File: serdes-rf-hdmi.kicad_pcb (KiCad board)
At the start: 4 copper layers, 33.5 x 33 mm, 13 parts, among them J1 HDMI_A, J2 SMA, J3 SMA

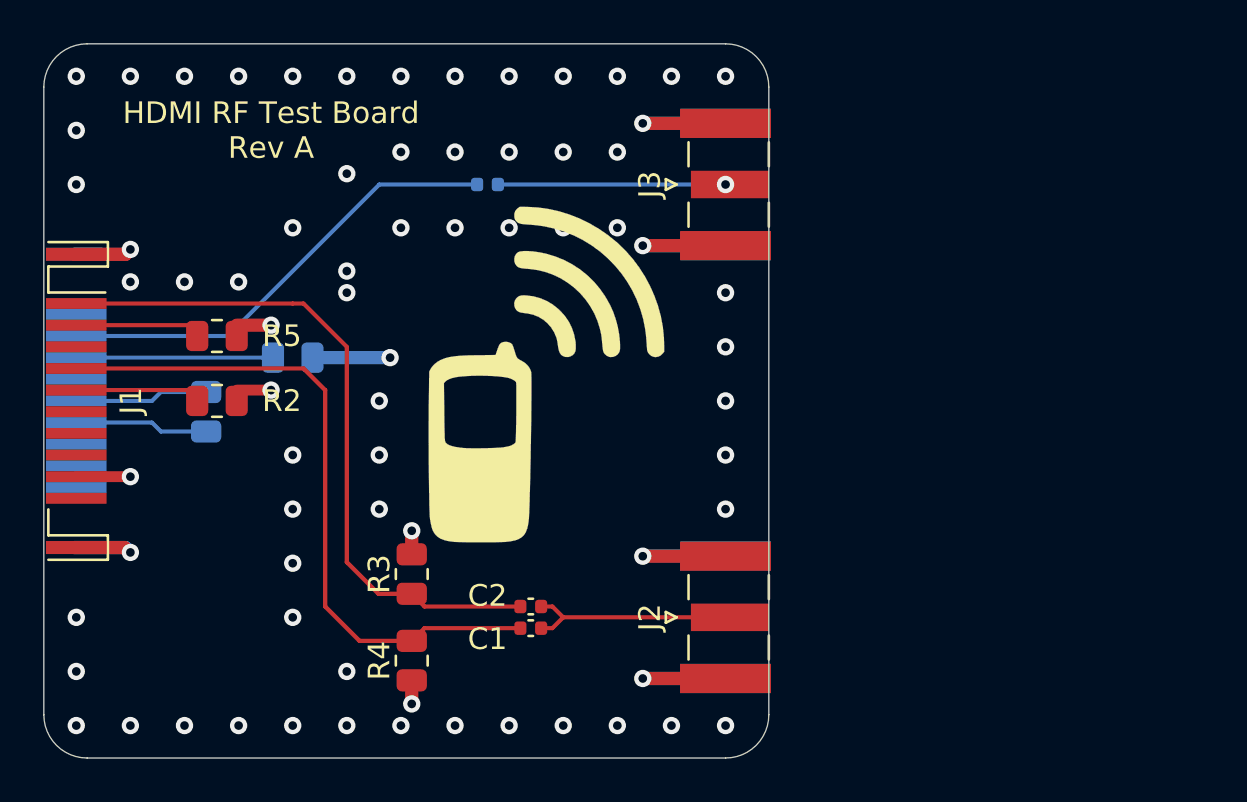
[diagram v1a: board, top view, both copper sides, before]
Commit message: Rev B complete
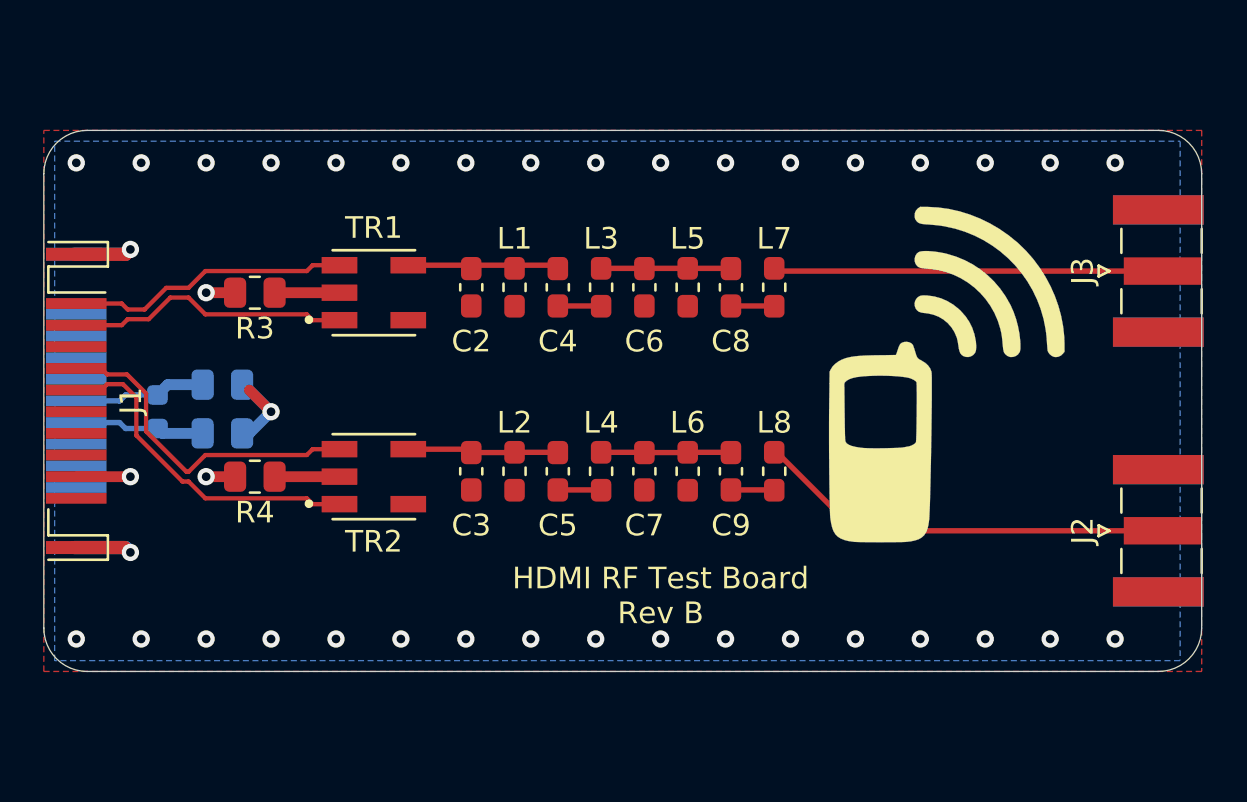
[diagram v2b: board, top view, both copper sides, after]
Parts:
- removed R5, R6: 50R, Resistor_SMD:R_0805_2012Metric
- added C4: 3.3pF, Capacitor_SMD:C_0603_1608Metric_Pad1.08x0.95mm_HandSolder, F.Cu at (142.2, 79.8)
- added C5: 3.3pF, Capacitor_SMD:C_0603_1608Metric_Pad1.08x0.95mm_HandSolder, F.Cu at (142.2, 88.2)
- added C6: 160pF, Capacitor_SMD:C_0603_1608Metric_Pad1.08x0.95mm_HandSolder, F.Cu at (146.2, 79.8)
- added C7: 160pF, Capacitor_SMD:C_0603_1608Metric_Pad1.08x0.95mm_HandSolder, F.Cu at (146.2, 88.2)
- added C8: 3.3pF, Capacitor_SMD:C_0603_1608Metric_Pad1.08x0.95mm_HandSolder, F.Cu at (150.2, 79.8)
- added C9: 3.3pF, Capacitor_SMD:C_0603_1608Metric_Pad1.08x0.95mm_HandSolder, F.Cu at (150.2, 88.2)
- added L1: 8.2nH, Inductor_SMD:L_0603_1608Metric_Pad1.05x0.95mm_HandSolder, F.Cu at (140.2, 79.8)
- added L2: 8.2nH, Inductor_SMD:L_0603_1608Metric_Pad1.05x0.95mm_HandSolder, F.Cu at (140.2, 88.2)
- added L3: 430nH, Inductor_SMD:L_0603_1608Metric_Pad1.05x0.95mm_HandSolder, F.Cu at (144.2, 79.8)
- added L4: 430nH, Inductor_SMD:L_0603_1608Metric_Pad1.05x0.95mm_HandSolder, F.Cu at (144.2, 88.2)
- added L5: 8.2nH, Inductor_SMD:L_0603_1608Metric_Pad1.05x0.95mm_HandSolder, F.Cu at (148.2, 79.8)
- added L6: 8.2nH, Inductor_SMD:L_0603_1608Metric_Pad1.05x0.95mm_HandSolder, F.Cu at (148.2, 88.2)
- added L7: 430nH, Inductor_SMD:L_0603_1608Metric_Pad1.05x0.95mm_HandSolder, F.Cu at (152.2, 79.8)
- added L8: 430nH, Inductor_SMD:L_0603_1608Metric_Pad1.05x0.95mm_HandSolder, F.Cu at (152.2, 88.2)
- added TR1: TC1-1TX+, serdes-rf-hdmi:XFMR_TC1-1-13M+, F.Cu at (133.8, 80.0)
- added TR2: TC1-1TX+, serdes-rf-hdmi:XFMR_TC1-1-13M+, F.Cu at (133.8, 88.5)
- C1: footprint Capacitor_SMD:C_0402_1005Metric -> Capacitor_SMD:C_0603_1608Metric; moved to B.Cu
- C2: value 10nF -> 160pF; footprint Capacitor_SMD:C_0402_1005Metric -> Capacitor_SMD:C_0603_1608Metric_Pad1.08x0.95mm_HandSolder
- C3: value 10nF -> 160pF; footprint Capacitor_SMD:C_0402_1005Metric -> Capacitor_SMD:C_0603_1608Metric_Pad1.08x0.95mm_HandSolder; moved to F.Cu
- R2: moved to B.Cu
- moved J2 25.6 mm to (170.0, 91.0)
- moved J3 25.6 mm to (170.0, 79.0)
- moved C1 19.9 mm to (123.8, 85.5), turned to 270 degrees
- moved G1 18.5 mm to (158.5, 84.0)
- moved C2 15.0 mm to (138.2, 79.8), turned to 270 degrees
- moved R3 14.9 mm to (128.2, 80.0), turned to 180 degrees
- moved C3 13.3 mm to (138.2, 88.2), turned to 270 degrees
- moved R4 11.2 mm to (128.2, 88.5), turned to 180 degrees
- moved R2 1.52 mm to (126.8, 86.5), turned to 180 degrees
- moved R1 1.46 mm to (126.8, 84.2), turned to 180 degrees
- renumbered J3 to J2, J2 to J3
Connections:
- C1 pad 2: /rfin- -> Net-(C1-Pad2)
- C2 pad 1: Net-(C1-Pad1) -> Net-(C2-Pad1)
- C2 pad 2: /rfin+ -> GND
- C3 pad 2: Net-(C3-Pad2) -> GND
- J1 pad 1: /rfin+ -> /rfa+
- J1 pad 10: Net-(J1-Pad10) -> Net-(C1-Pad1)
- J1 pad 12: Net-(J1-Pad12) -> Net-(C1-Pad2)
- J1 pad 3: Net-(J1-Pad3) -> /rfa-
- J1 pad 4: Net-(C3-Pad2) -> Net-(J1-Pad4)
- J1 pad 7: /rfin- -> /rfb+
- J1 pad 9: Net-(J1-Pad9) -> /rfb-
- J2 pad 1: Net-(C3-Pad1) -> Net-(J2-Pad1)
- J3 pad 1: Net-(C1-Pad1) -> Net-(J3-Pad1)
- R1 pad 1: Net-(J1-Pad10) -> GND
- R1 pad 2: Net-(J1-Pad12) -> Net-(C1-Pad1)
- R2 pad 1: Net-(J1-Pad9) -> GND
- R2 pad 2: GND -> Net-(C1-Pad2)
- R3 pad 1: /rfin+ -> Net-(R3-Pad1)
- R4 pad 1: /rfin- -> Net-(R4-Pad1)
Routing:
- net /rfin+: track 32.1 -> 0.00 mm
- net GND: track 52.8 -> 21.0 mm, vias 72 -> 40
- net /rfin-: track 31.8 -> 0.00 mm
- net Net-(C3-Pad2): track 21.4 -> 0.00 mm
- net Net-(J2-Pad1): track 0.00 -> 19.5 mm
- net Net-(J3-Pad1): track 0.00 -> 18.1 mm
- net /rfb-: track 0.00 -> 15.6 mm
- net /rfb+: track 0.00 -> 15.6 mm
- net /rfa-: track 0.00 -> 13.1 mm
- net /rfa+: track 0.00 -> 13.1 mm
- net Net-(J1-Pad6): track 9.09 -> 0.00 mm
- net Net-(C2-Pad1): track 0.00 -> 6.98 mm
- net Net-(J1-Pad12): track 6.17 -> 0.00 mm
- net Net-(J1-Pad10): track 6.17 -> 0.00 mm
- net Net-(C1-Pad2): track 0.00 -> 6.04 mm
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- added copper zone on B.Cu, net GND
- added copper zone on F.Cu, net GND
- removed copper zone on F.Cu, net (none)
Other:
- board size 33.5 x 33 mm -> 53.5 x 25 mm
- board text added: "HDMI RF Test Board Rev B"
- board text removed: "HDMI RF Test Board Rev A"
